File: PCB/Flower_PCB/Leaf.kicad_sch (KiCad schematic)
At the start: 17 parts, among them J7 Conn_01x02_Pin

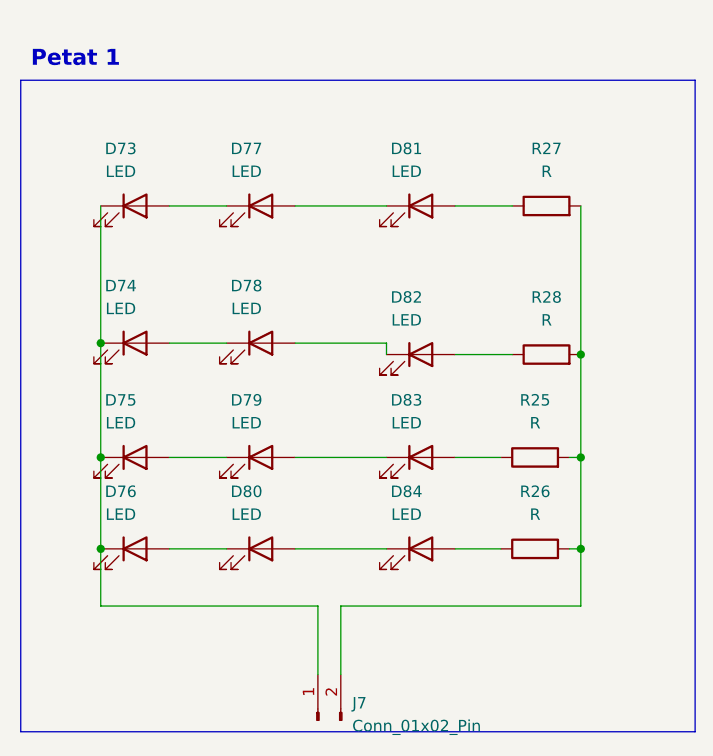
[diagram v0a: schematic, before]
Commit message: the petal designe has been updated
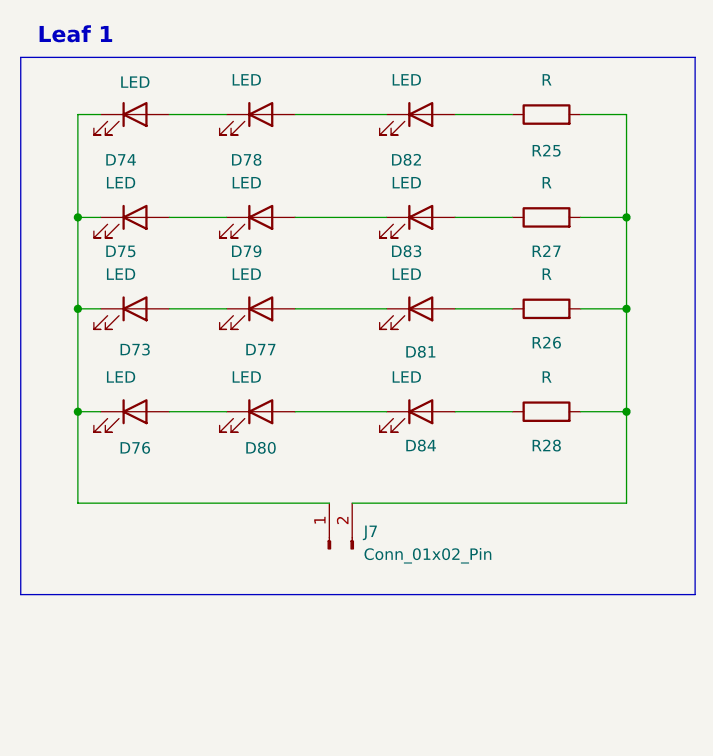
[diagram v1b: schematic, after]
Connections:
- net at D84.2 (A): now also R28.1; no longer R26.1
- net at D83.2 (A): now also R27.1; no longer R25.1
- net at D82.2 (A): now also R26.1; no longer R28.1
- net at D81.2 (A): now also R25.1; no longer R27.1
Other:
- note added: "Leaf 1"
- note removed: "Petat 1"
